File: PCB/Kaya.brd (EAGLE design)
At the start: 34 x 30 mm, 23 parts, among them U1 MCP73832T-2ACI/OT, U2 LSM9DS1

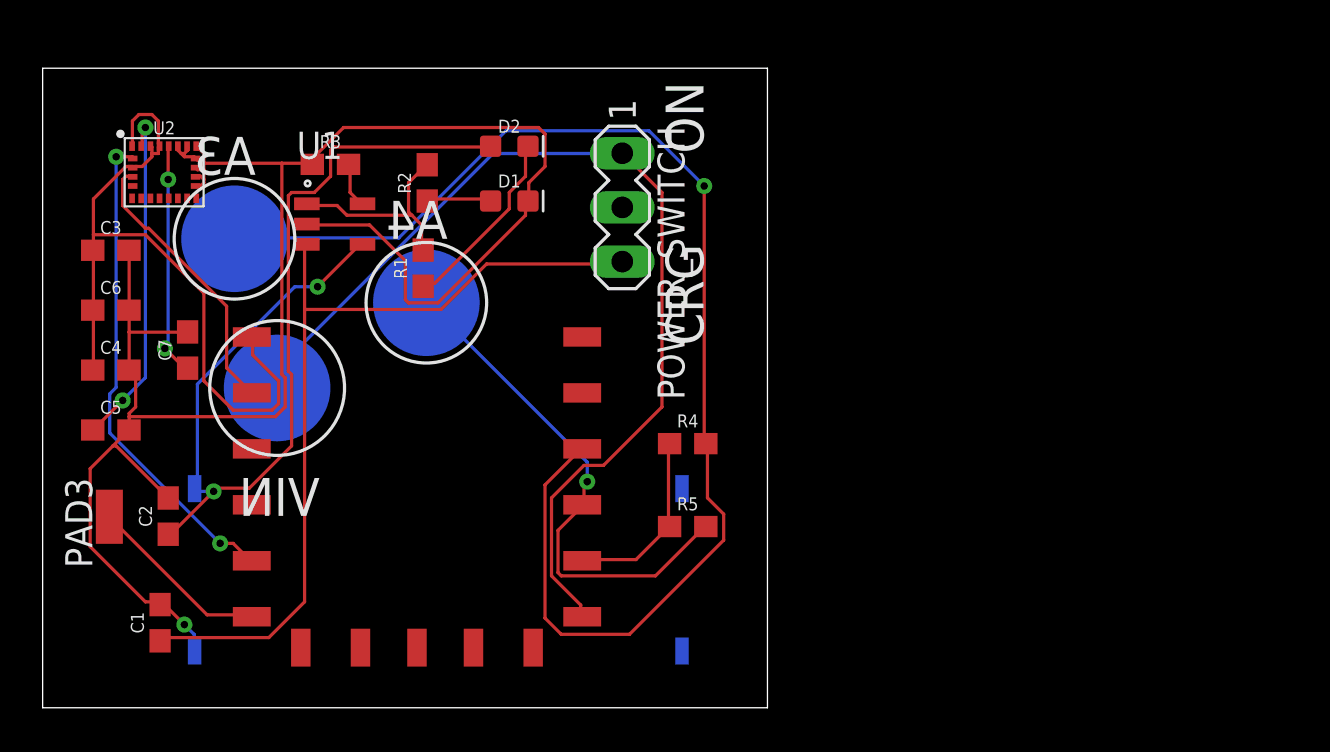
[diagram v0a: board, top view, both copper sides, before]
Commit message: Finished PCB
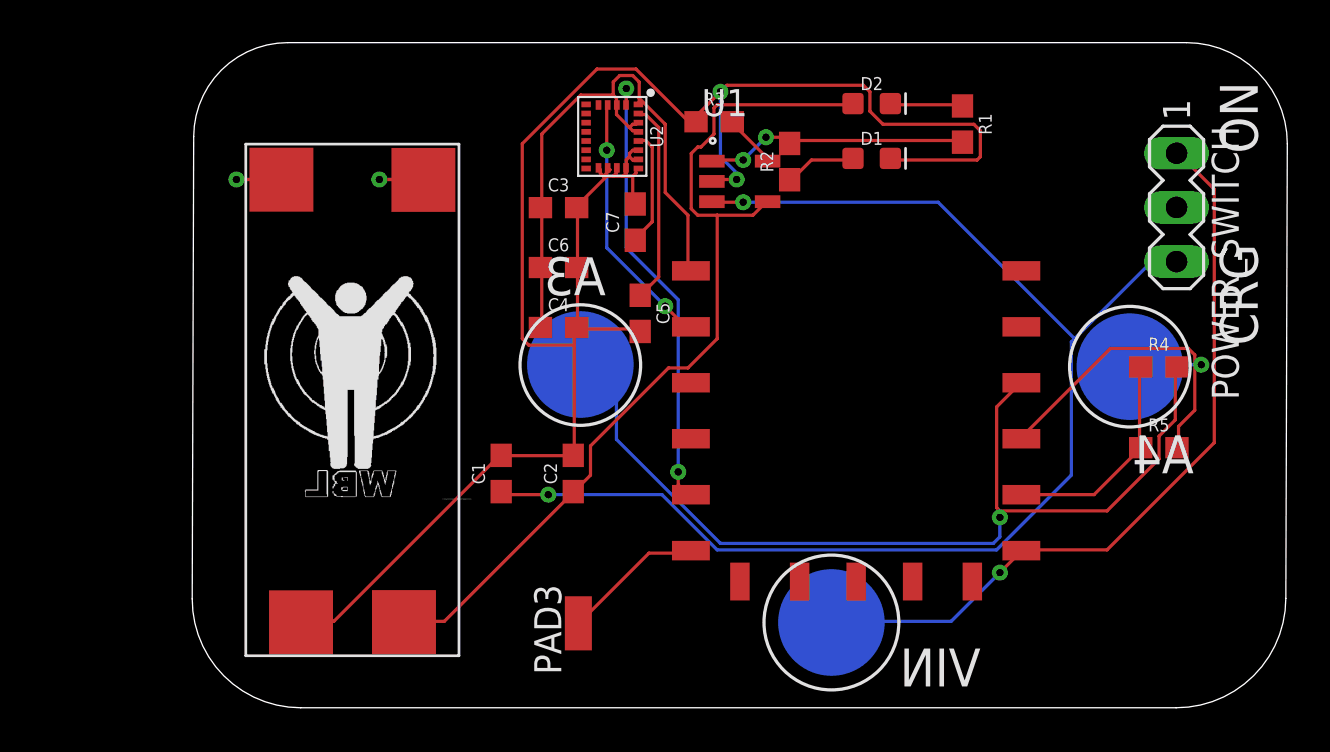
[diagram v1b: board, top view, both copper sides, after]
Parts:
- added PAD1, PAD2: WIREPADSMD1,27-254, wirepad:SMD1,27-2,54
- moved U$4 33.1 mm to (57.0, 63.0)
- moved U$5 28.2 mm to (43.0, 51.0)
- moved R1 26.2 mm to (49.1, 74.4), turned to 270 degrees
- moved POWER_SWITCH 26.0 mm to (59.2, 70.5)
- moved C5 25.4 mm to (34.0, 65.5), turned to 270 degrees
- moved PAD3 22.6 mm to (31.1, 51.0)
- moved R5 22.4 mm to (58.4, 59.2)
- moved R4 22.4 mm to (58.4, 63.0)
- moved C7 21.8 mm to (33.8, 69.8)
- moved C3 21.1 mm to (30.2, 70.5)
- moved C4 21.1 mm to (30.2, 64.8)
- moved C6 21.1 mm to (30.2, 67.7)
- moved U2 21.1 mm to (32.7, 73.8), turned to 270 degrees
- moved U$2 20.8 mm to (44.2, 57.9)
- moved U1 19.1 mm to (38.7, 71.7)
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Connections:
- new net N$10: PAD1.1, U$1.IN_R
- new net N$11: PAD2.1, U$1.IN_L
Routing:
- net VBAT: track 40.3 -> 61.8 mm, vias 0 -> 2
- net N$4: track 61.4 -> 46.1 mm
- net VIN: track 47.1 -> 35.8 mm, vias 0 -> 1
- net N$12: track 16.2 -> 9.46 mm, vias 2 -> 0
- net VDD: track 35.0 -> 28.5 mm
- net N$6: track 24.4 -> 18.4 mm
- net N$14: track 11.0 -> 5.48 mm, vias 2 -> 0
- net N$7: track 8.90 -> 3.41 mm
- net N$2: track 46.9 -> 42.6 mm, vias 2 -> 0
- net N$11: track 0.00 -> 4.13 mm, vias 0 -> 1
- net N$10: track 0.00 -> 4.01 mm, vias 0 -> 1
- net N$8: track 9.81 -> 12.5 mm, vias 0 -> 2
- net N$5: track 8.62 -> 6.68 mm
- net N$17: track 23.1 -> 21.2 mm
- net N$3: track 8.67 -> 10.3 mm
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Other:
- board size 34 x 30 mm -> 51.4 x 31.2 mm
- board text added: "C:/Users/mcons/Downloads/kTq6gCz2.bmp"
